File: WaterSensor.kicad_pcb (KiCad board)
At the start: 2 copper layers, 25.4 x 51.4 mm, 3 parts, among them U1 NRF9160-DK

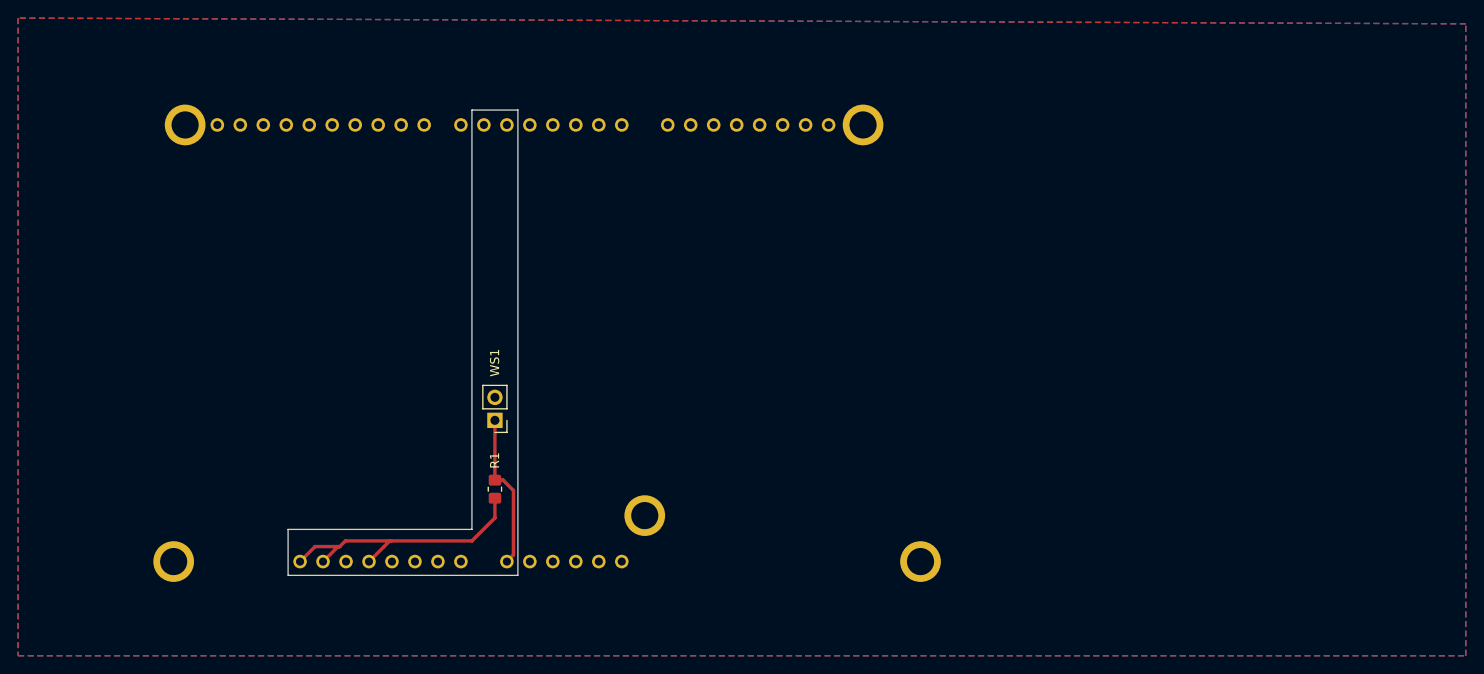
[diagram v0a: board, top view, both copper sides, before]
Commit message: board v1.0
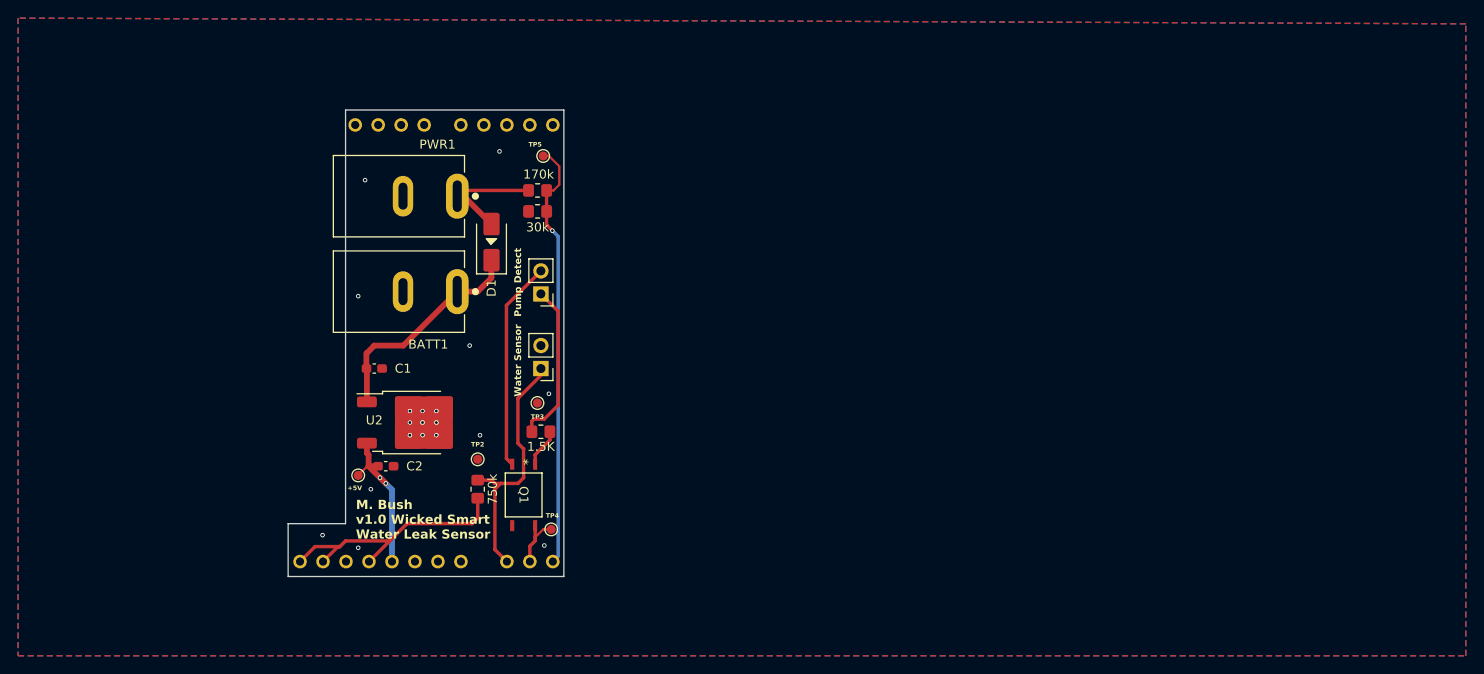
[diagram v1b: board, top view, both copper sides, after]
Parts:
- added BATT1: PJ-037A, PJ-037A:CUI_PJ-037A, F.Cu at (122.8, 74.0)
- added C1: 1uF, Capacitor_SMD:C_0603_1608Metric_Pad1.08x0.95mm_HandSolder, F.Cu at (113.7, 82.5)
- added C2: 1uF, Capacitor_SMD:C_0603_1608Metric_Pad1.08x0.95mm_HandSolder, F.Cu at (114.9, 93.3)
- added D1: US1G, Diode_SMD:D_SMA, F.Cu at (126.6, 68.6)
- added PD1: Conn_01x02, Connector_PinHeader_2.54mm:PinHeader_1x02_P2.54mm_Vertical, F.Cu at (132.1, 74.3)
- added PWR1: PJ-037A, PJ-037A:CUI_PJ-037A, F.Cu at (122.8, 63.5)
- added Q1: 140357145200, footprints:WL-OCPT_SOP4_WRE, F.Cu at (130.2, 96.5)
- added R2: 170k, Resistor_SMD:R_0805_2012Metric_Pad1.20x1.40mm_HandSolder, F.Cu at (131.7, 62.9)
- added R3: 30k, Resistor_SMD:R_0805_2012Metric_Pad1.20x1.40mm_HandSolder, F.Cu at (131.7, 65.2)
- added R4: 1.5K, Resistor_SMD:R_0805_2012Metric_Pad1.20x1.40mm_HandSolder, F.Cu at (132.1, 89.5)
- added TP1: TestPoint, TestPoint:TestPoint_Pad_D1.0mm, F.Cu at (111.9, 94.4)
- added TP2: TestPoint, TestPoint:TestPoint_Pad_D1.0mm, F.Cu at (125.1, 92.6)
- added TP3: TestPoint, TestPoint:TestPoint_Pad_D1.0mm, F.Cu at (131.7, 86.4)
- added TP4: TestPoint, TestPoint:TestPoint_Pad_D1.0mm, F.Cu at (133.2, 100.3)
- added TP5: TestPoint, TestPoint:TestPoint_Pad_D1.0mm, F.Cu at (132.3, 59.1)
- added U2: BD50FC0FP, Package_TO_SOT_SMD:TO-252-2, F.Cu at (117.9, 88.5)
- R1: value 1M -> 750k
- moved WS1 7.66 mm to (132.1, 82.5)
- moved R1 1.91 mm to (125.1, 95.9)
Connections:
- U1 pad P1_5: unconnected-(U1-P1_5V-PadP1_5) -> +5V
- U1 pad P2_2: unconnected-(U1-P2_P0.15_VCOM2_CTS-PadP2_2) -> PumpDetect
- U1 pad P2_3: unconnected-(U1-P2_P0.16/AIN3-PadP2_3) -> PowerDetect
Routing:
- net PowerDetect: track 0.00 -> 47.7 mm, vias 0 -> 1
- net +BATT: track 0.00 -> 24.6 mm
- net Net-(PD1-Pin_2): track 0.00 -> 23.2 mm
- net Net-(PD1-Pin_1): track 0.00 -> 17.9 mm
- net +5V: track 0.00 -> 17.7 mm, vias 0 -> 2
- net +12V: track 0.00 -> 13.2 mm
- net Net-(U1-P2_P0.14_VCOM2_RTS): track 17.3 -> 28.3 mm
- net PumpDetect: track 0.00 -> 6.36 mm
- net Net-(Q1-Pad1): track 0.00 -> 4.27 mm
- net Net-(R1-Pad1): track 31.7 -> 29.7 mm
- net GND: vias 0 -> 19
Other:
- board size 25.4 x 51.4 mm -> 30.5 x 51.6 mm
- board text added: "M. Bush v1.0 Wicked Smart Water Leak Sensor"
